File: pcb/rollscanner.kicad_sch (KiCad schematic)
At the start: 21 parts, among them J1 DIN-5, Q0 Q_NPN, Q1 Q_Photo_NPN, Q2 Q_Photo_NPN, Q3 Q_Photo_NPN, Q4 Q_Photo_NPN, U1 STM32G431C8Tx, U2 ADG706BRUZ, U3 ADG706BRUZ, U4 ADG706BRUZ, U5 ADG706BRUZ, U6 ADG706BRUZ, U7 ADG706BRUZ, U8 ADG706BRUZ

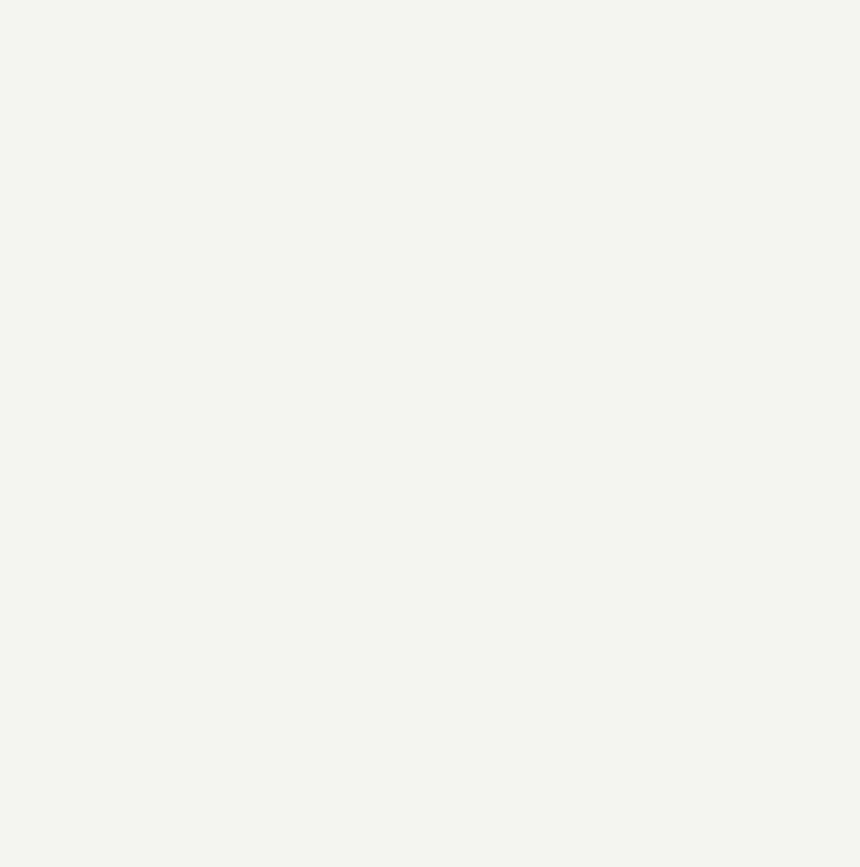
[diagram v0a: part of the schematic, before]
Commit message: a
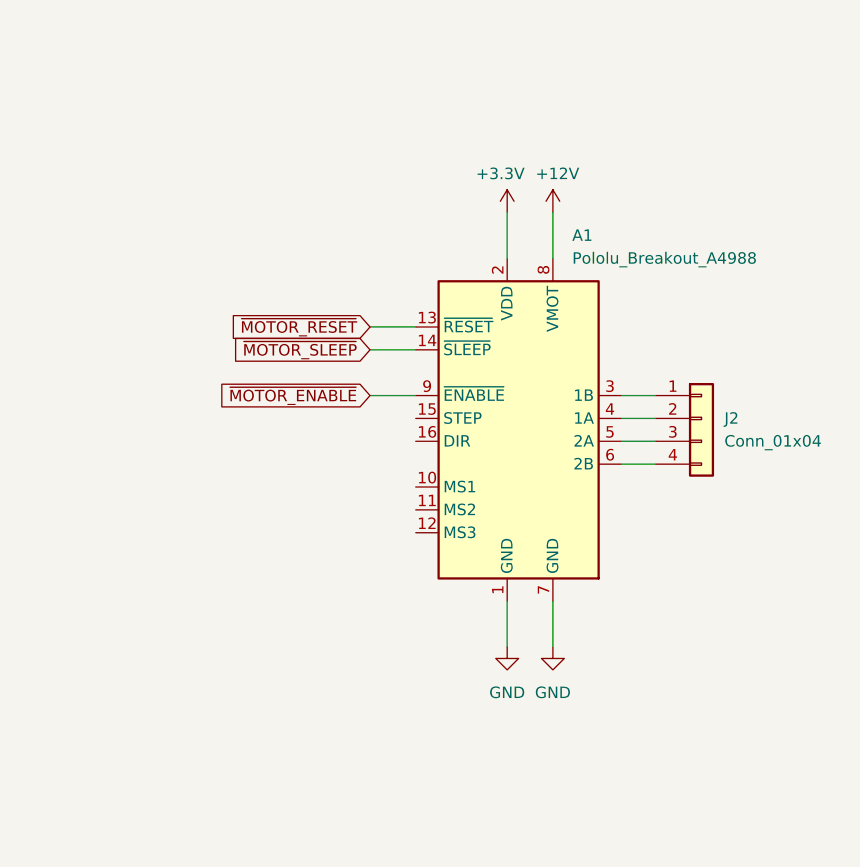
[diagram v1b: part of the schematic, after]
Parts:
- added A1: Pololu_Breakout_A4988, Module:Pololu_Breakout-16_15.2x20.3mm, symbol Driver_Motor:Pololu_Breakout_A4988
- added J2: Conn_01x04, symbol Connector_Generic:Conn_01x04
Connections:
- net +3.3V: now also A1.2 (VDD)
- net GND: now also A1.1 (GND), A1.7 (GND)
- new net: A1.3 (1B), J2.1 (Pin_1)
- new net: A1.4 (1A), J2.2 (Pin_2)
- new net: A1.5 (2A), J2.3 (Pin_3)
- new net: A1.6 (2B), J2.4 (Pin_4)
- new net +12V: A1.8 (VMOT)
- new net ~{MOTOR_ENABLE}: A1.9 (~{ENABLE})
- new net ~{MOTOR_RESET}: A1.13 (~{RESET})
- new net ~{MOTOR_SLEEP}: A1.14 (~{SLEEP})
